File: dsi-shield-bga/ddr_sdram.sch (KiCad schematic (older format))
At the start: 15 parts, among them IC10 MT46V32M16P-5B:F

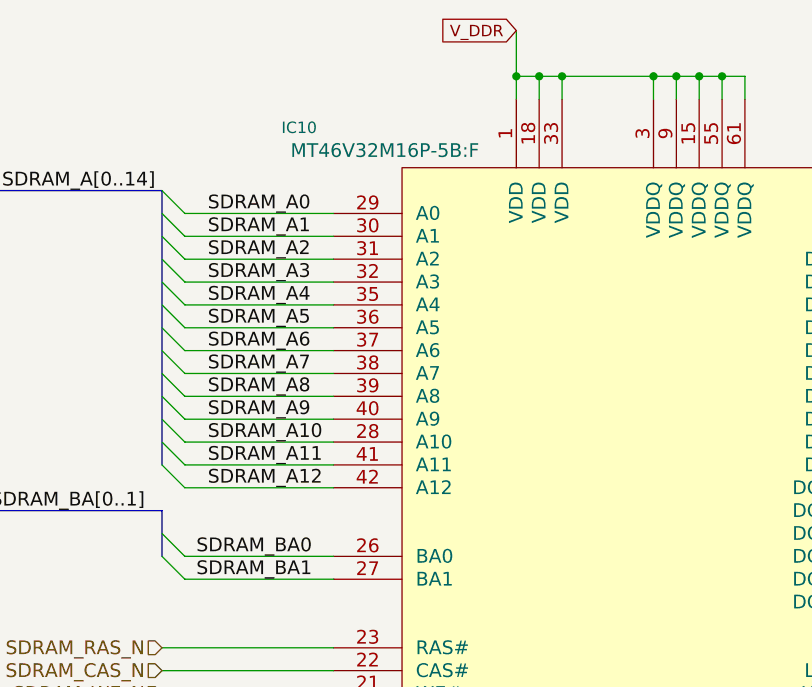
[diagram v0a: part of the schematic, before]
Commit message: pin head
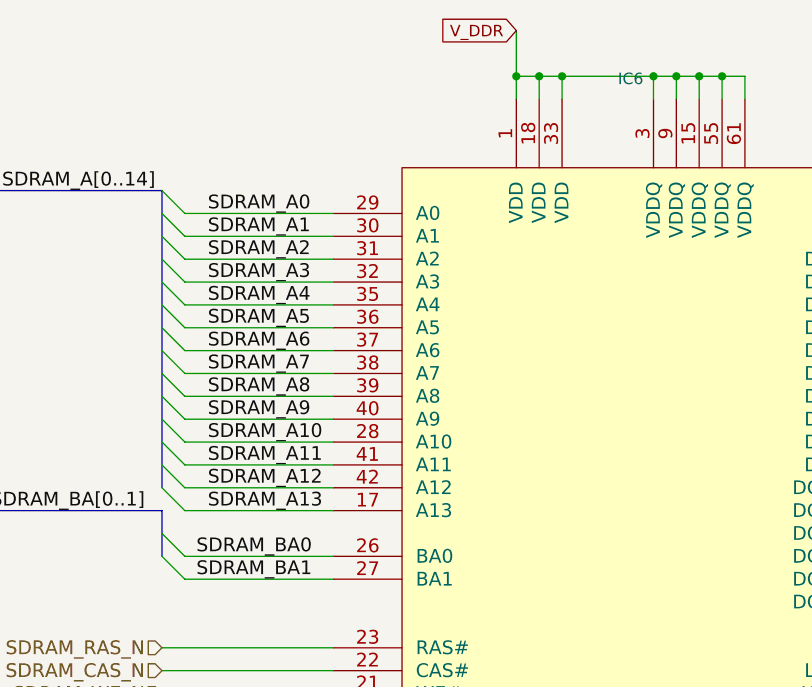
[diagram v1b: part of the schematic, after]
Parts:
- removed IC10: MT46V32M16P-5B:F, dsi_shield:TSOP66, symbol dsi_shield:MT46V32M16P-5B_F
- added IC6: MT46V64M16P-5B_F, dsi_shield:TSOP66, symbol mybays_memory:MT46V64M16P-5B_F
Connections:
- net DDR_VREF: now also IC6.49 (VREF)
- net GND: now also IC6.12 (VSSQ), IC6.34 (VSS), IC6.48 (VSS), IC6.52 (VSSQ), IC6.58 (VSSQ), IC6.6 (VSSQ), IC6.64 (VSSQ), IC6.66 (VSS)
- net SDRAM_A0: now also IC6.29 (A0)
- net SDRAM_A1: now also IC6.30 (A1)
- net SDRAM_A10: now also IC6.28 (A10)
- net SDRAM_A11: now also IC6.41 (A11)
- net SDRAM_A12: now also IC6.42 (A12)
- net SDRAM_A2: now also IC6.31 (A2)
- net SDRAM_A3: now also IC6.32 (A3)
- net SDRAM_A4: now also IC6.35 (A4)
- net SDRAM_A5: now also IC6.36 (A5)
- net SDRAM_A6: now also IC6.37 (A6)
- net SDRAM_A7: now also IC6.38 (A7)
- net SDRAM_A8: now also IC6.39 (A8)
- net SDRAM_A9: now also IC6.40 (A9)
- net SDRAM_BA0: now also IC6.26 (BA0)
- net SDRAM_BA1: now also IC6.27 (BA1)
- net SDRAM_CAS_N: now also IC6.22 (CAS#)
- net SDRAM_CKE: now also IC6.44 (CKE)
- net SDRAM_CLK_N: now also IC6.46 (CK#)
- net SDRAM_CLK_P: now also IC6.45 (CK)
- net SDRAM_CS_N: now also IC6.24 (CS#)
- net SDRAM_DQ0: now also IC6.2 (DQ0)
- net SDRAM_DQ1: now also IC6.4 (DQ1)
- net SDRAM_DQ10: now also IC6.57 (DQ10)
- net SDRAM_DQ11: now also IC6.59 (DQ11)
- net SDRAM_DQ12: now also IC6.60 (DQ12)
- net SDRAM_DQ13: now also IC6.62 (DQ13)
- net SDRAM_DQ14: now also IC6.63 (DQ14)
- net SDRAM_DQ15: now also IC6.65 (DQ15)
- net SDRAM_DQ2: now also IC6.5 (DQ2)
- net SDRAM_DQ3: now also IC6.7 (DQ3)
- net SDRAM_DQ4: now also IC6.8 (DQ4)
- net SDRAM_DQ5: now also IC6.10 (DQ5)
- net SDRAM_DQ6: now also IC6.11 (DQ6)
- net SDRAM_DQ7: now also IC6.13 (DQ7)
- net SDRAM_DQ8: now also IC6.54 (DQ8)
- net SDRAM_DQ9: now also IC6.56 (DQ9)
- net SDRAM_DQM0: now also IC6.20 (LDM)
- net SDRAM_DQM1: now also IC6.47 (UDM)
- net SDRAM_DQS0: now also IC6.16 (LDQS)
- net SDRAM_DQS1: now also IC6.51 (UDQS)
- net SDRAM_RAS_N: now also IC6.23 (RAS#)
- net SDRAM_WE_N: now also IC6.21 (WE#)
- net V_DDR: now also IC6.1 (VDD), IC6.15 (VDDQ), IC6.18 (VDD), IC6.3 (VDDQ), IC6.33 (VDD), IC6.55 (VDDQ), IC6.61 (VDDQ), IC6.9 (VDDQ)
- new net SDRAM_A13: IC6.17 (A13)
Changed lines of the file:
@@
 Comment4 ""
 $EndDescr
-$Comp
-L dsi_shield:MT46V32M16P-5B_F IC10
-U 1 1 59956E83
-P 7650 4450
-F 0 "IC10" H 4500 7425 50  0000 C CNN
-F 1 "MT46V32M16P-5B:F" H 4875 7325 60  0000 C CNN
-F 2 "dsi_shield:TSOP66" H 7650 3400 60  0001 L CNN
-F 3 "" H 7650 3310 60  0001 L CNN
-F 4 "Value" H 7650 4450 60  0001 C CNN "Fieldname"
-F 5 "MT46V32M16P-5B:F" H 7650 3220 60  0001 L CNN "Field4"
-F 6 "Yes" H 7650 3130 60  0001 L CNN "Field5"
-F 7 "MT46V32M16P-5B:F" H 7650 3040 60  0001 L CNN "Field6"
-	1    7650 4450
-	1    0    0    -1
-$EndComp
 Text Label 4100 1850 0    60   ~ 0
 SDRAM_A0
@@
 Wire Wire Line
 	3900 4750 4650 4750
+$Comp
+L mybays_memory:MT46V64M16P-5B_F IC6
+U 1 1 5F2E917C
+P 7650 4450
+F 0 "IC6" H 5950 7639 50  0000 C CNN
+F 1 "MT46V64M16P-5B_F" H 7650 3490 60  0001 L CNN
+F 2 "dsi_shield:TSOP66" H 7650 3400 60  0001 L CNN
+F 3 "" H 7650 3310 60  0001 L CNN
+F 4 "MT46V32M16P-5B:F" H 7650 3220 60  0001 L CNN "Field4"
+F 5 "Yes" H 7650 3130 60  0001 L CNN "Field5"
+F 6 "MT46V32M16P-5B:F" H 7650 3040 60  0001 L CNN "Field6"
+	1    7650 4450
+	1    0    0    -1
+$EndComp
+Wire Wire Line
+	4000 3150 4650 3150
+Entry Wire Line
+	4000 3150 3900 3050
+Text Label 4100 3150 0    60   ~ 0
+SDRAM_A13
 Wire Bus Line
 	3900 3150 3900 3350
@@
 	8200 4350 8200 4500
 Wire Bus Line
-	3900 1750 3900 2950
+	3900 1750 3900 3050
 Wire Bus Line
 	8200 2150 8200 3750
